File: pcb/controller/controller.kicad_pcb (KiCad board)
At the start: 2 copper layers, 94.4 x 89.8 mm, 1 part, among them U1 Pico

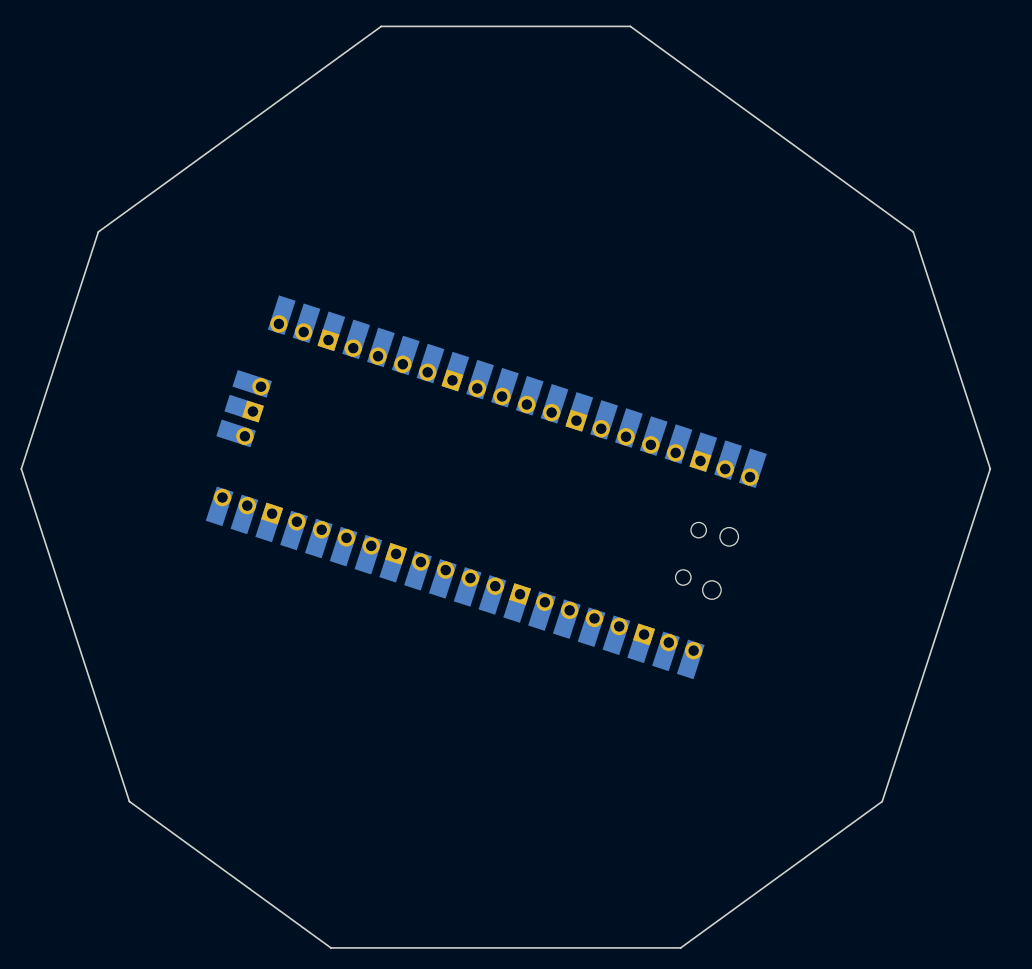
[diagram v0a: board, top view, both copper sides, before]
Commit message: Checkpoint after controller gerbers.
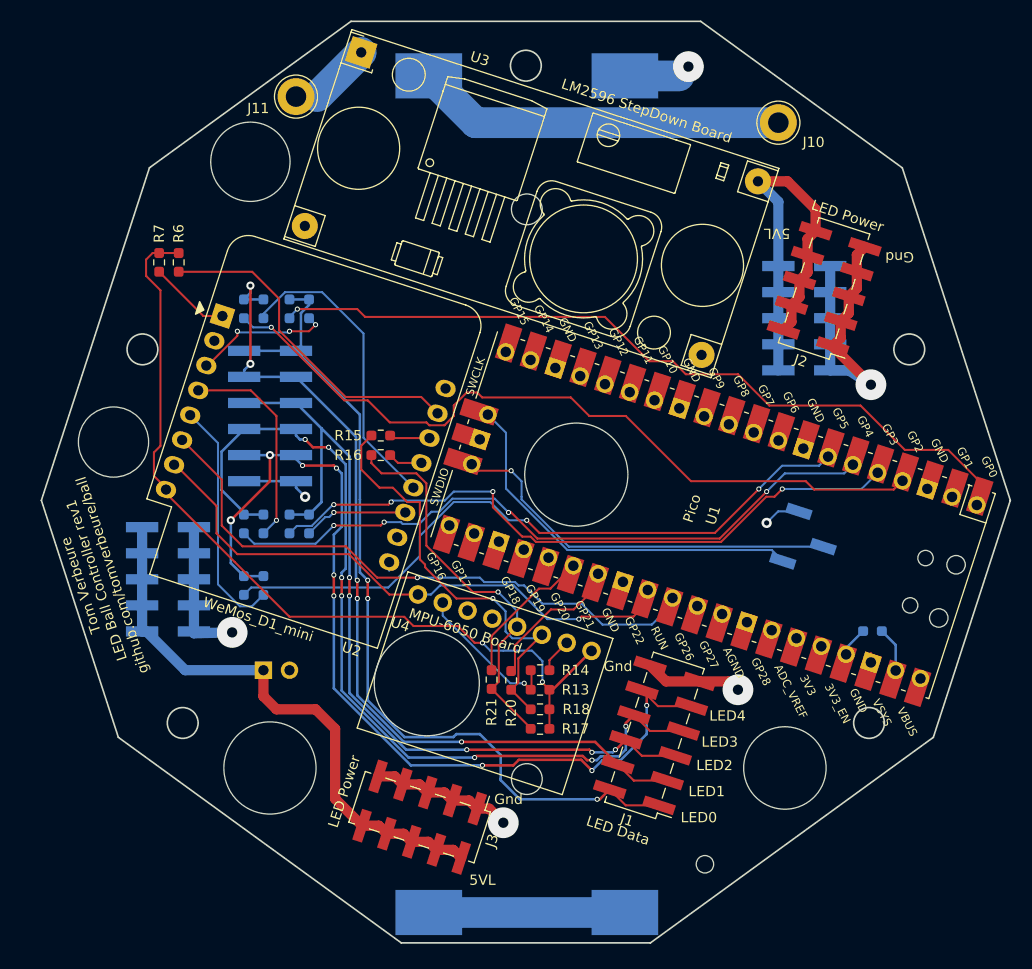
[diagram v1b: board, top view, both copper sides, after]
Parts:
- added BT1: Battery_Two_Cell, 2x18650_battery_holder:battery_holder, B.Cu at (153.9, 85.1)
- added J1: LED Data, Connector_PinHeader_2.54mm:PinHeader_2x06_P2.54mm_Vertical_SMD, F.Cu at (166.4, 108.6)
- added J10: Conn_01x01, TestPoint:TestPoint_Loop_D3.80mm_Drill2.0mm, F.Cu at (178.4, 48.9)
- added J11: Conn_01x01, TestPoint:TestPoint_Loop_D3.80mm_Drill2.0mm, F.Cu at (131.4, 46.4)
- added J2: LED Power, Connector_PinHeader_2.54mm:PinHeader_2x05_P2.54mm_Vertical_SMD, F.Cu at (182.9, 65.0)
- added J3: LED Power, Connector_PinHeader_2.54mm:PinHeader_2x05_P2.54mm_Vertical_SMD, F.Cu at (143.5, 116.6)
- added J4: LED Power, Connector_PinHeader_2.54mm:PinHeader_2x05_P2.54mm_Vertical_SMD, B.Cu at (119.0, 93.4)
- added J5: locked, Connector_PinHeader_2.54mm:PinHeader_2x05_P2.54mm_Vertical_SMD, B.Cu at (181.0, 67.9)
- added J6: LED Data, Connector_PinHeader_2.54mm:PinHeader_2x06_P2.54mm_Vertical_SMD, B.Cu at (128.9, 77.5)
- added J7: Conn_01x03_Male, Connector_PinHeader_2.54mm:PinHeader_1x03_P2.54mm_Vertical_SMD_Pin1Left, B.Cu at (181.2, 89.7)
- added JP1: 5V Power, Connector_PinHeader_2.54mm:PinHeader_1x02_P2.54mm_Vertical, B.Cu at (128.3, 102.2)
- added R1: R, Resistor_SMD:R_0603_1608Metric_Pad0.98x0.95mm_HandSolder, B.Cu at (132.7, 67.0)
- added R10: R, Resistor_SMD:R_0603_1608Metric_Pad0.98x0.95mm_HandSolder, B.Cu at (126.4, 88.0)
- added R11: R, Resistor_SMD:R_0603_1608Metric_Pad0.98x0.95mm_HandSolder, B.Cu at (128.3, 94.0)
- added R12: R, Resistor_SMD:R_0603_1608Metric_Pad0.98x0.95mm_HandSolder, B.Cu at (126.4, 94.0)
- added R13: R, Resistor_SMD:R_0603_1608Metric_Pad0.98x0.95mm_HandSolder, F.Cu at (155.2, 104.1)
- added R14: R, Resistor_SMD:R_0603_1608Metric_Pad0.98x0.95mm_HandSolder, F.Cu at (155.2, 102.2)
- added R15: 100K, Resistor_SMD:R_0603_1608Metric_Pad0.98x0.95mm_HandSolder, F.Cu at (139.7, 79.4)
- added R16: 100K, Resistor_SMD:R_0603_1608Metric_Pad0.98x0.95mm_HandSolder, F.Cu at (139.7, 81.3)
- added R17: R, Resistor_SMD:R_0603_1608Metric_Pad0.98x0.95mm_HandSolder, F.Cu at (155.2, 108.0)
- added R18: R, Resistor_SMD:R_0603_1608Metric_Pad0.98x0.95mm_HandSolder, F.Cu at (155.2, 106.0)
- added R19: 100K, Resistor_SMD:R_0603_1608Metric_Pad0.98x0.95mm_HandSolder, B.Cu at (187.6, 98.4)
- added R2: R, Resistor_SMD:R_0603_1608Metric_Pad0.98x0.95mm_HandSolder, B.Cu at (130.8, 67.0)
- added R20: 100K, Resistor_SMD:R_0603_1608Metric_Pad0.98x0.95mm_HandSolder, F.Cu at (152.4, 103.2)
- added R21: 100K, Resistor_SMD:R_0603_1608Metric_Pad0.98x0.95mm_HandSolder, F.Cu at (150.5, 103.1)
- added R3: R, Resistor_SMD:R_0603_1608Metric_Pad0.98x0.95mm_HandSolder, B.Cu at (128.3, 67.0)
- added R4: R, Resistor_SMD:R_0603_1608Metric_Pad0.98x0.95mm_HandSolder, B.Cu at (126.4, 67.0)
- added R5: R, Resistor_SMD:R_0603_1608Metric_Pad0.98x0.95mm_HandSolder, B.Cu at (132.7, 88.0)
- added R6: R, Resistor_SMD:R_0603_1608Metric_Pad0.98x0.95mm_HandSolder, F.Cu at (120.0, 62.5)
- added R7: R, Resistor_SMD:R_0603_1608Metric_Pad0.98x0.95mm_HandSolder, F.Cu at (118.1, 62.5)
- added R8: R, Resistor_SMD:R_0603_1608Metric_Pad0.98x0.95mm_HandSolder, B.Cu at (130.8, 88.0)
- added R9: R, Resistor_SMD:R_0603_1608Metric_Pad0.98x0.95mm_HandSolder, B.Cu at (128.3, 88.0)
- added U2: WeMos_D1_mini, Module:WEMOS_D1_mini_light, F.Cu at (124.3, 67.7)
- added U3: LM2596 StepDown Board, LM2596_Board:YAAJ_DCDC_StepDown_LM2596, F.Cu at (137.8, 42.1)
- added U4: MPU-6050 Board, MPU-6050_Board:MPU-6050_Board_no_screw_holes, F.Cu at (149.9, 103.5)
- U1: moved to F.Cu
- moved U1 22.3 mm to (172.1, 87.1), turned to -108 degrees
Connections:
- U1 pad 1: unconnected-(U1-Pad1) -> /LED0_PICO
- U1 pad 18: unconnected-(U1-Pad18) -> GND
- U1 pad 23: unconnected-(U1-Pad23) -> GND
- U1 pad 26: unconnected-(U1-Pad26) -> Net-(R21-Pad2)
- U1 pad 27: unconnected-(U1-Pad27) -> Net-(R20-Pad2)
- U1 pad 28: unconnected-(U1-Pad28) -> GND
- U1 pad 29: unconnected-(U1-Pad29) -> /INT
- U1 pad 3: unconnected-(U1-Pad3) -> GND
- U1 pad 30: unconnected-(U1-Pad30) -> /PICO_RUN
- U1 pad 37: unconnected-(U1-Pad37) -> Net-(R19-Pad2)
- U1 pad 38: unconnected-(U1-Pad38) -> GND
- U1 pad 39: unconnected-(U1-Pad39) -> Net-(R19-Pad1)
- U1 pad 4: unconnected-(U1-Pad4) -> /LED1_PICO
- U1 pad 40: unconnected-(U1-Pad40) -> +5V
- U1 pad 41: unconnected-(U1-Pad41) -> /SWCLK
- U1 pad 42: unconnected-(U1-Pad42) -> GND
- U1 pad 43: unconnected-(U1-Pad43) -> /SWDIO
- U1 pad 5: unconnected-(U1-Pad5) -> /LED2_PICO
- U1 pad 6: unconnected-(U1-Pad6) -> /LED3_PICO
- U1 pad 7: unconnected-(U1-Pad7) -> /LED4_PICO
- U1 pad 8: unconnected-(U1-Pad8) -> GND
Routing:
- net +5VL: track 0.00 -> 96.3 mm
- net /LED4: track 0.00 -> 93.2 mm, vias 0 -> 9
- net GND: track 0.00 -> 92.6 mm, vias 0 -> 7
- net /LED3: track 0.00 -> 86.1 mm, vias 0 -> 7
- net /LED1: track 0.00 -> 84.8 mm, vias 0 -> 5
- net /LED0: track 0.00 -> 84.5 mm, vias 0 -> 3
- net +3V3: track 0.00 -> 83.4 mm, vias 0 -> 2
- net /LED2: track 0.00 -> 81.5 mm, vias 0 -> 5
- net /LED0_PICO: track 0.00 -> 76.8 mm, vias 0 -> 1
- net /LED1_PICO: track 0.00 -> 74.7 mm, vias 0 -> 1
- net +5V: track 0.00 -> 74.4 mm
- net /LED3_PICO: track 0.00 -> 66.3 mm, vias 0 -> 4
- net /LED4_PICO: track 0.00 -> 66.1 mm, vias 0 -> 2
- net /LED2_PICO: track 0.00 -> 64.7 mm, vias 0 -> 4
- net /PICO_RUN: track 0.00 -> 59.3 mm, vias 0 -> 1
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- added copper zone on In2.Cu, net +5VL
- added copper zone on In1.Cu, net GND
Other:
- outline, holes or cut-outs redrawn
- copper layers 2 -> 4
- board text added: "5VL"
- board text added: "GND"
- board text added: "Gnd"
- board text added: "LED0"
- board text added: "LED1"
- board text added: "LED2"
- board text added: "LED3"
- board text added: "LED4"
- board text added: "SWCLK"
- board text added: "SWDIO"
- board text added: "Tom Verbeure LED Ball Controller rev1 github.com/tomverbeure/ball"
